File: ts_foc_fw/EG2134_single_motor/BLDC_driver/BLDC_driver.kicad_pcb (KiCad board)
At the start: 2 copper layers, 85.5 x 76 mm, 56 parts, among them CN1 XT30PW-M, CN2 MR30PW-M30.G.Y, CN3 WAFER-GH1.25-10PWB, Q1 RU3089M-C, Q2 RU3089M-C, Q3 RU3089M-C, Q4 RU3089M-C, Q5 RU3089M-C, Q6 RU3089M-C, U1 EG2134_N, U2 TPS54331DDAR, U3 INA240A2PW, U4 INA240A2PW

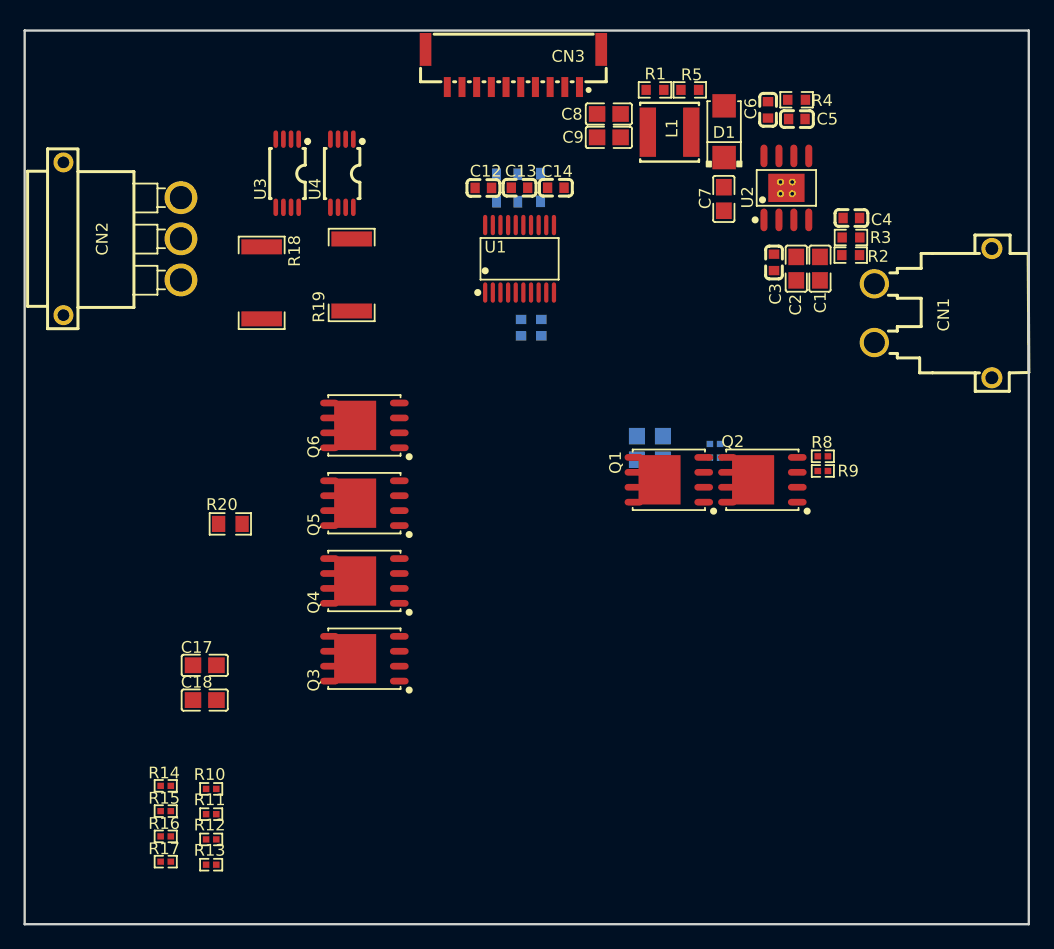
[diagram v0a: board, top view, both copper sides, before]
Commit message: 同步
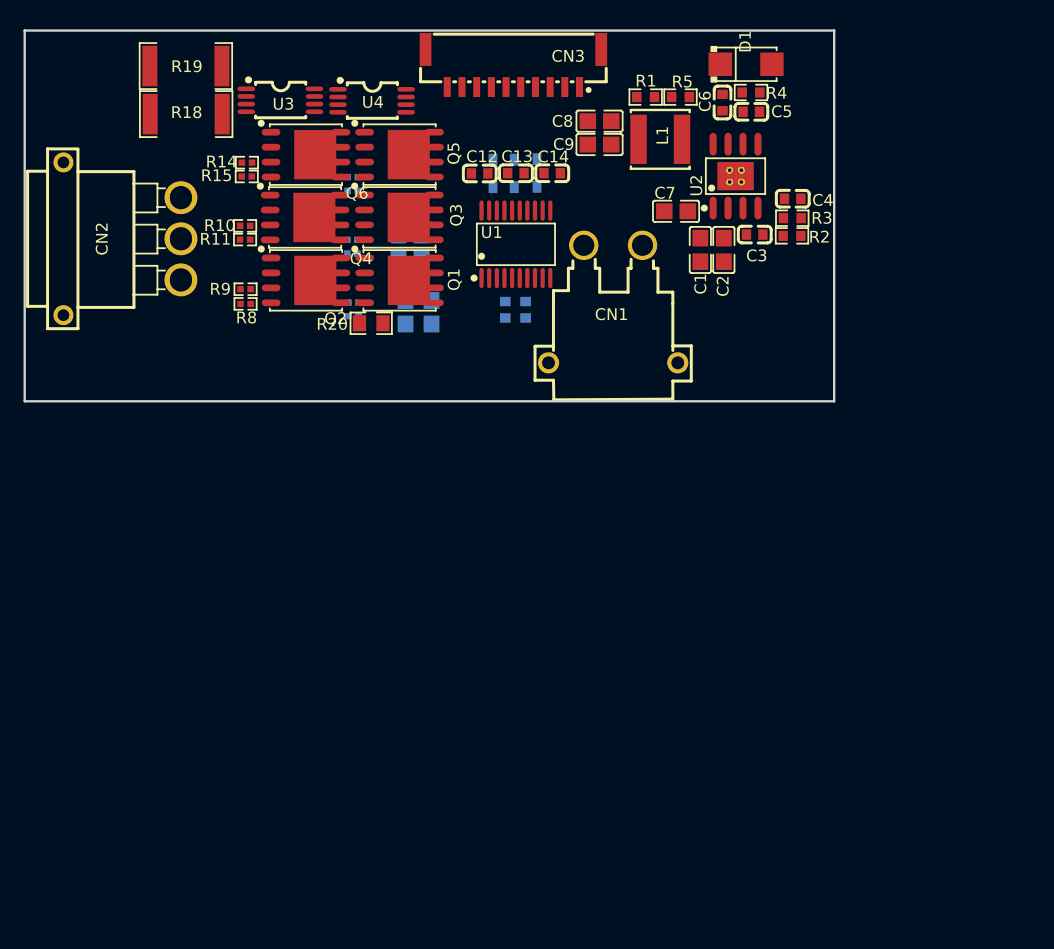
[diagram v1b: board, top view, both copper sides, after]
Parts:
- C17, C18, R12, R13, R16, R17: moved to B.Cu
- moved R17 59.3 mm to (49.5, 31.4), turned to 180 degrees
- moved R16 58.3 mm to (49.5, 30.3)
- moved R15 54.4 mm to (40.5, 30.2)
- moved R14 53.5 mm to (40.5, 29.0), turned to 180 degrees
- moved R13 53.4 mm to (49.5, 36.8), turned to 180 degrees
- moved R12 52.4 mm to (49.5, 35.6)
- moved R9 51.5 mm to (40.4, 39.8), turned to 0 degrees
- moved R8 50.8 mm to (40.4, 41.0), turned to 180 degrees
- moved R11 49.0 mm to (40.3, 35.6)
- moved R10 48.0 mm to (40.4, 34.4), turned to 180 degrees
- moved Q2 42.4 mm to (45.5, 39.0), turned to -90 degrees
- moved C18 42.0 mm to (53.4, 36.2), turned to -90 degrees
- moved C17 40.1 mm to (55.4, 36.2), turned to -90 degrees
- moved Q3 37.7 mm to (53.5, 33.7), turned to -90 degrees
- moved R7 33.5 mm to (49.6, 40.9), turned to 0 degrees
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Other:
- board size 85.5 x 76 mm -> 68.9 x 31.5 mm
